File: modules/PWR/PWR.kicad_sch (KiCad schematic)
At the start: 18 parts, among them SW1 POWER ON, SW2 RESET, U1 74HC00

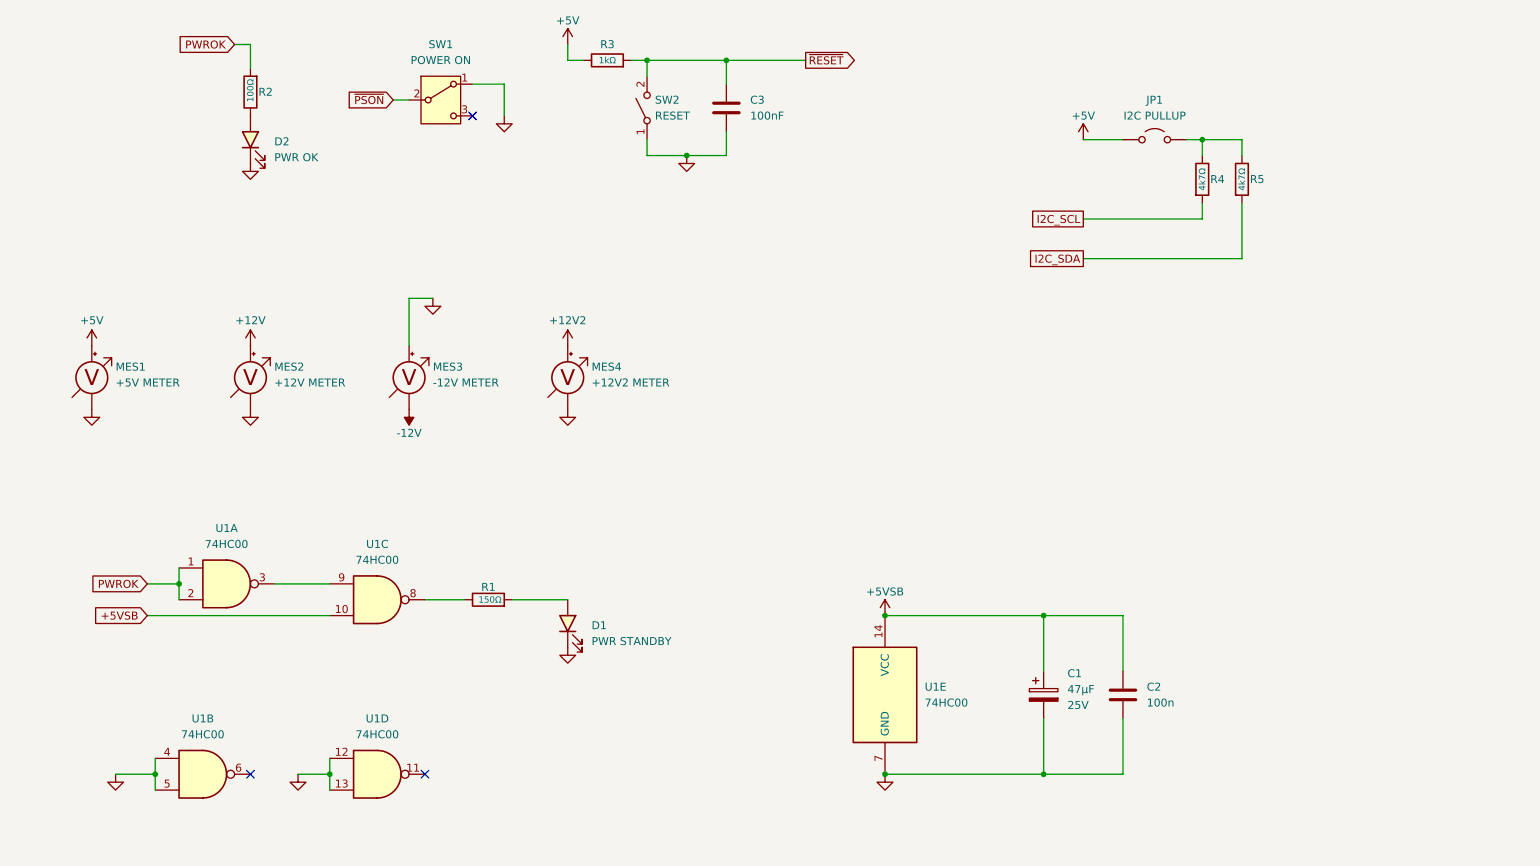
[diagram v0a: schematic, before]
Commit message: pwr pcb
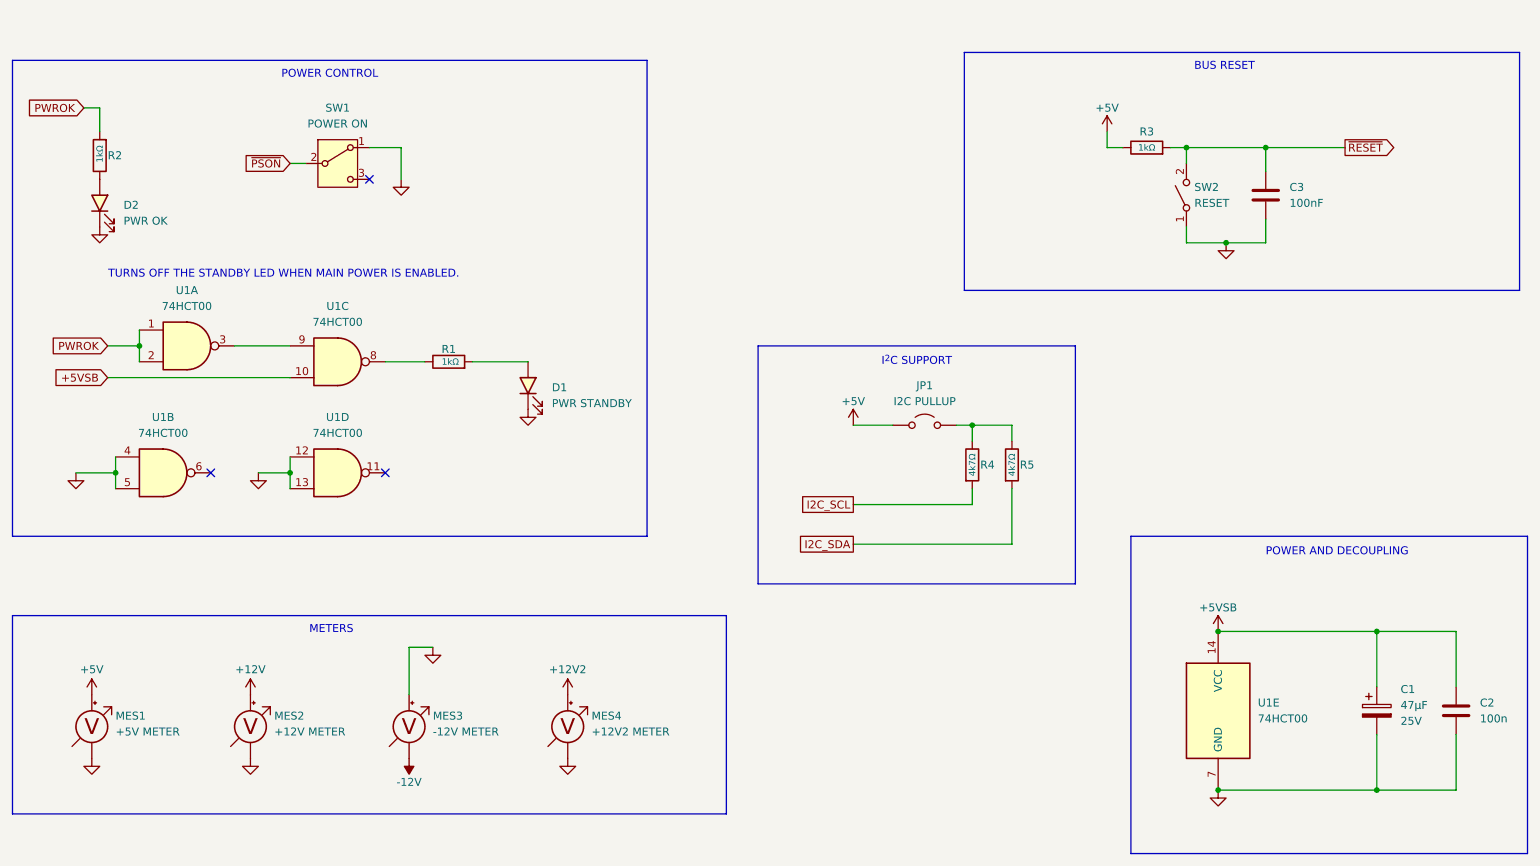
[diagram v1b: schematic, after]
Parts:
- R1: value 150Ω -> 1kΩ
- R2: value 100Ω -> 1kΩ
- U1: value 74HC00 -> 74HCT00
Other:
- note added: "BUS RESET"
- note added: "I^{2}C SUPPORT"
- note added: "METERS"
- note added: "POWER AND DECOUPLING"
- note added: "POWER CONTROL"
- note added: "TURNS OFF THE STANDBY LED WHEN MAIN POWER IS ENABLED."
- title: PWR-CTRL -> PWR
- moved on the sheet: C1, C2, C3, D1, D2, JP1, MES1, MES2, MES3, MES4, R1, R2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
